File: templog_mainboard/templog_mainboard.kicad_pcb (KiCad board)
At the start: 4 copper layers, 57 parts, among them J1 USB_C_Receptacle_USB2.0_16P, J3 battery_con, Q1 Si1308EDL, U1 ESP32-S3-MINI-1, U2 DS3231MZ, U3 SHT4x, U4 BQ27441-G1, U5 BQ24075RGT, U6 24LC512, U7 USBLC6-2SC6, U8 ADP2303ARDZ-3.3

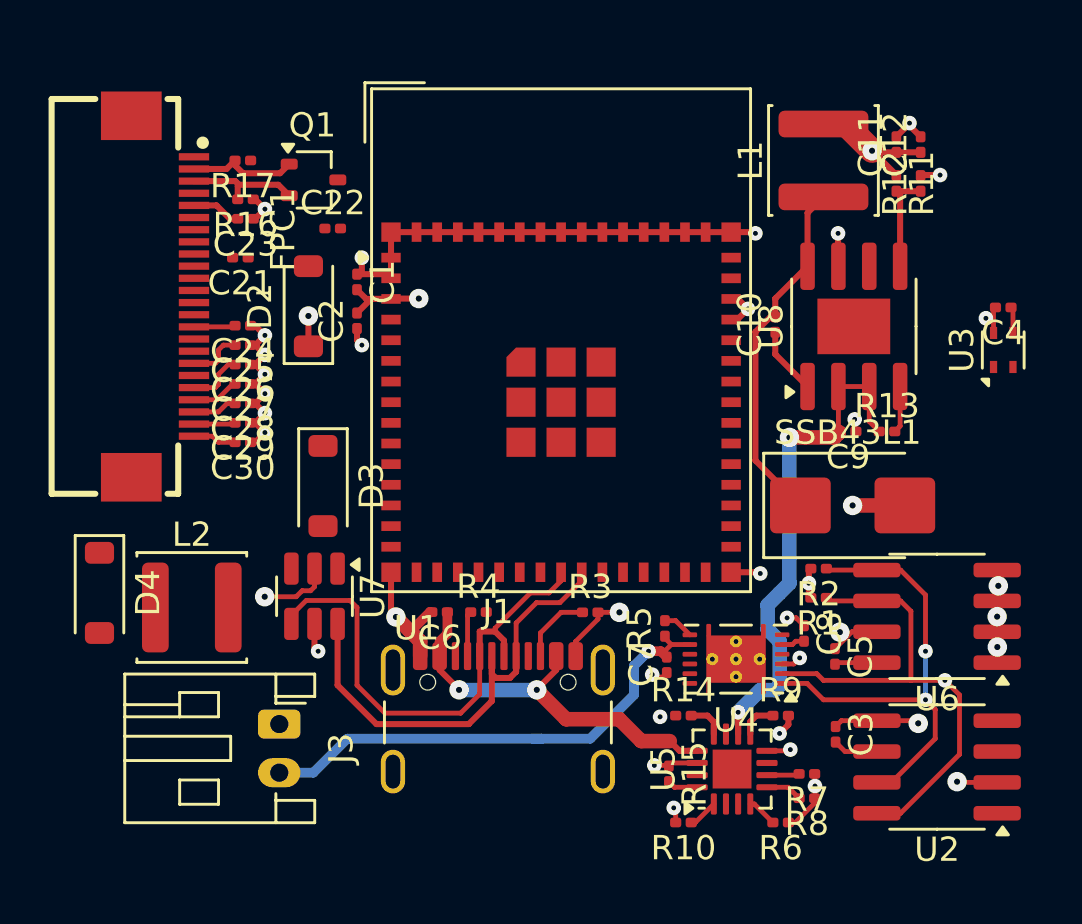
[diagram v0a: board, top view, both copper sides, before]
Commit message: electiricity
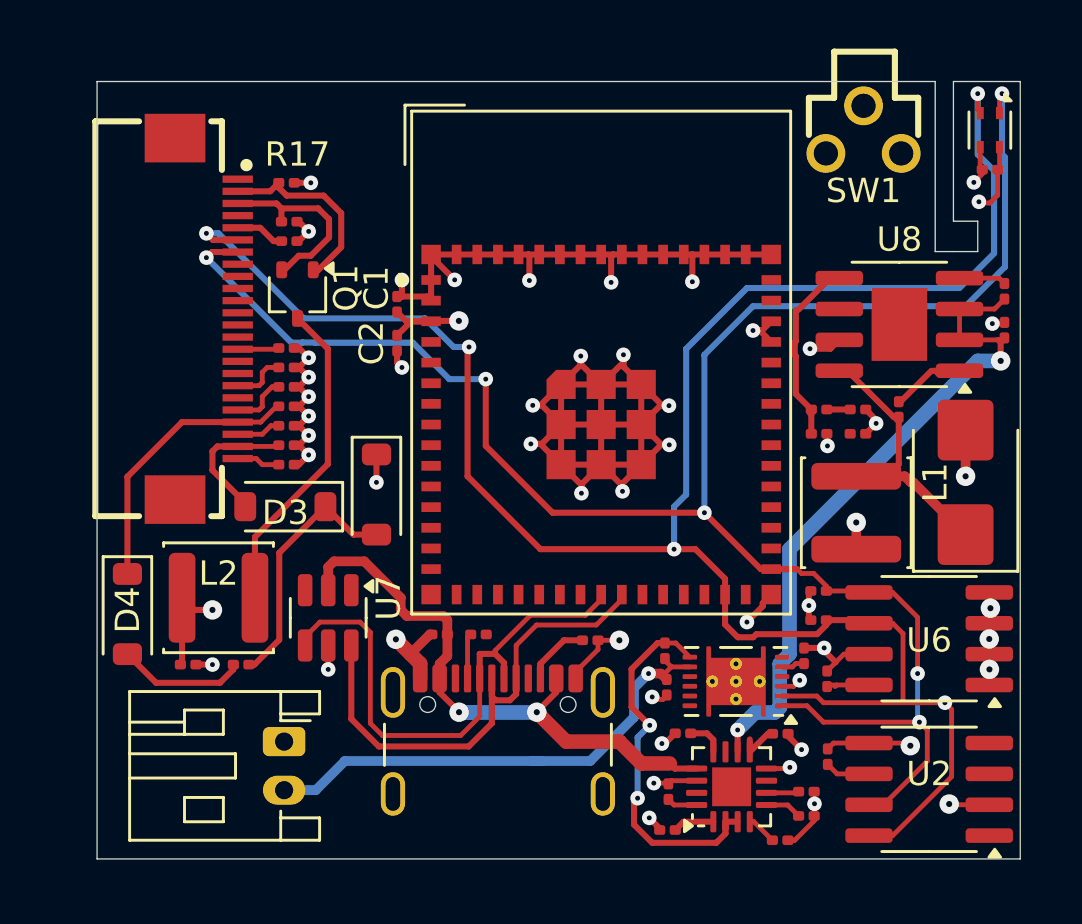
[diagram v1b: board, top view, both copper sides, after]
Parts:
- added SW1: K2-1109DE-D4SW-01, K2-1109DE-D4SW-01:KEY-TH_K2-1109DE-CXXW-XX, F.Cu at (161.1, 41.7)
- moved C22 18.3 mm to (135.4, 63.8), turned to 180 degrees
- moved C21 16.9 mm to (133.2, 63.8), turned to 0 degrees
- moved L1 14.6 mm to (160.8, 57.5), turned to -90 degrees
- moved C12 12.2 mm to (160.8, 54.2), turned to 0 degrees
- moved R12 11.1 mm to (159.2, 54.2), turned to 0 degrees
- moved C11 11.0 mm to (160.8, 53.2), turned to 0 degrees
- moved R11 9.83 mm to (159.2, 53.2), turned to 180 degrees
- moved U3 9.07 mm to (166.2, 41.8), turned to -90 degrees
- moved D2 8.24 mm to (141.0, 56.8), turned to -90 degrees
- moved C9 7.67 mm to (166.8, 50.0), turned to -90 degrees
- moved R13 7.53 mm to (166.8, 48.4), turned to 90 degrees
- moved C10 6.17 mm to (162.5, 53.2), turned to -90 degrees
- moved C4 5.69 mm to (166.3, 43.4), turned to 0 degrees
- moved Q1 4.75 mm to (137.8, 48.5), turned to -90 degrees
- moved SSB43L1 4.75 mm to (165.2, 56.2), turned to 90 degrees
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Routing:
- net /I2C_SCL: track 22.4 -> 90.7 mm, vias 1 -> 5
- net /I2C_SDA: track 20.7 -> 82.7 mm, vias 2 -> 6
- net GND: track 66.3 -> 116.3 mm, vias 36 -> 48
- net Net-(D4-A): track 0.00 -> 20.1 mm
- net /power_mgmt/V_battery: track 1.27 -> 15.6 mm, vias 0 -> 2
- net Net-(D2-A): track 0.00 -> 10.5 mm
- net /PREVGH: track 1.96 -> 11.4 mm
- net +3.3V: track 17.1 -> 24.1 mm, vias 4 -> 6
- net /power_mgmt/powerpath_out: track 21.2 -> 27.7 mm
- net /power_mgmt/+5VUSB: track 19.2 -> 24.5 mm, vias 3 -> 2
- net Net-(U8-FB): track 4.11 -> 8.26 mm
- net /PREVGL: track 1.71 -> 5.67 mm
- net /GDR: track 4.56 -> 8.00 mm
- net /RESE: track 4.79 -> 7.91 mm
- net Net-(SSB43L1-K): track 14.7 -> 12.5 mm
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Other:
- board outline added: 38 x 32 mm
